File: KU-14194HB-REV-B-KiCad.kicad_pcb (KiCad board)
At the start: 2 copper layers, 388.6 x 180.3 mm, 220 parts, among them CN1 KEYBOARD_20PIN_MALE, CN10 LED_CONNECTOR, CN2 USER_PORT_CON, CN3 CASSETTE_PORT_CON, CN4 SERIAL_BUS_CON, CN5 AV_CONN, CN6 EXPANSION_PORT, CN7 POWER_CON, CN8 CONTROL_PORT, CN9 CONTROL_PORT, M1 MODULATOR_LONGBOARD, Q1 2SC1815, Q2 2SC1815, Q3 TP298/2SD880, Q7 2SC1815, Q8 2SC1815, SW1 POWER_SWITCH, U1 CIA_U1, U10 4164-2, U11 4164-2, U12 4164-2, U13 74LS257, U14 74LS258, U15 74LS139, U16 4066_U28, U17 PLA_U17, U18 6581, U19 VIC, U2 CIA_U2, U20 556, U21 4164-2, U22 4164-2, U23 4164-2, U24 4164-2, U25 74LS257, U26 74LS373, U27 7408_U27, U28 4066_U28, U29 74LS74, U3 2364A, U30 74LS193, U31 74LS629N, U32 MC4044, U4 2364A, U5 2332A, U6 2114, U7 6510_MPU, U8 7406N, U9 4164-2, Y1 Crystal

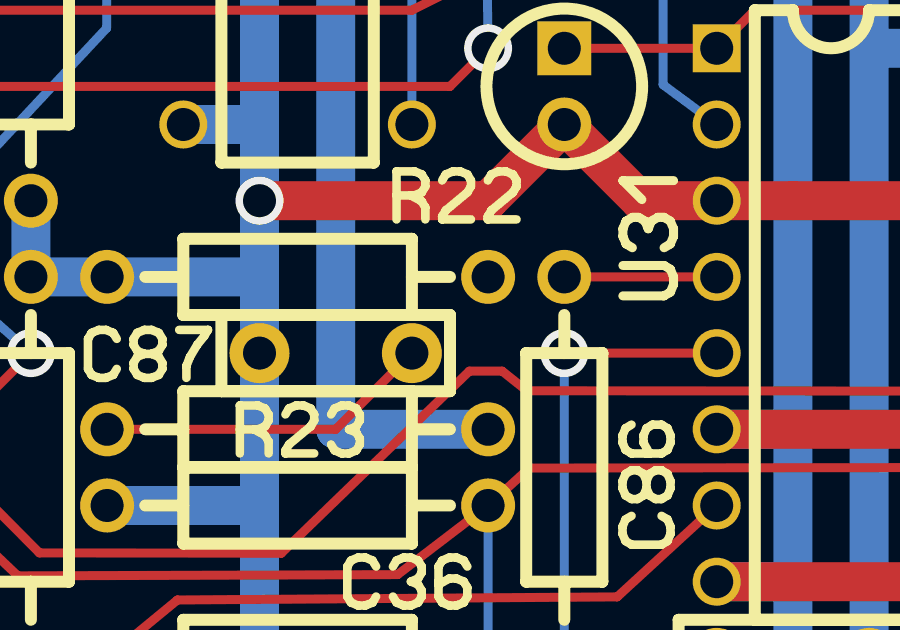
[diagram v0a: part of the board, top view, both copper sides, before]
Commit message: Update V1.3
See readme
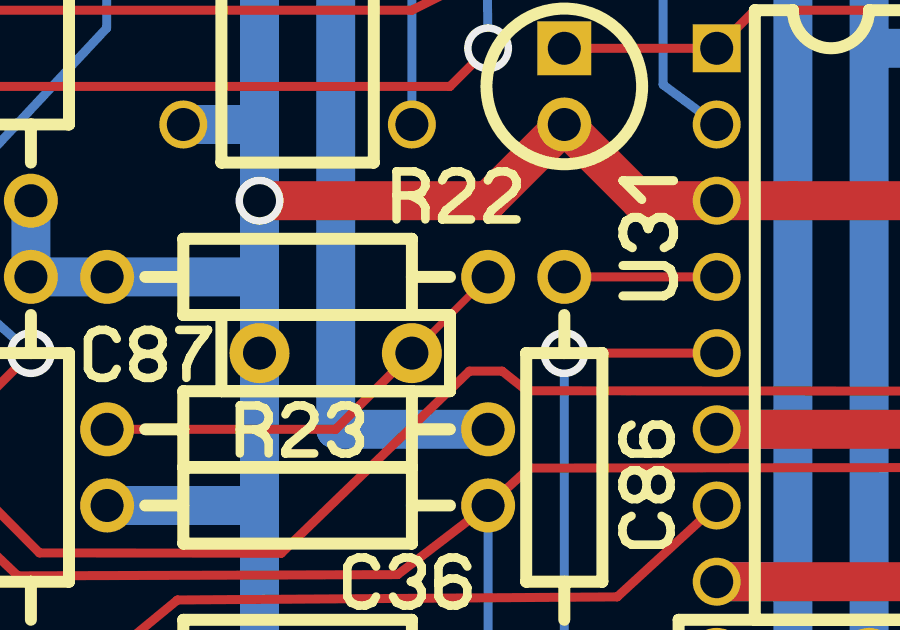
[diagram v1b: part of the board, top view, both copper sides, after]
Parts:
- C36: value .1 -> 20pF
- C86: value ? -> 82pF
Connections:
- R22 pad 1: Net-(R22-Pad1) -> Net-(C87-Pad1)
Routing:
- net Net-(C87-Pad1): track 11.2 -> 14.8 mm
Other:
- board text added: "Replica 1.3 by BWACK 2019"
- board text removed: "Replica 1.1 by BWACK 2019"
